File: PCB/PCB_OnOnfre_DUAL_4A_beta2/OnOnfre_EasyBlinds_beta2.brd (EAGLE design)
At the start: 44.4 x 46 mm, 27 parts, among them J3Y S8050, J7 8p, K1 OMRON-G3MB-202P-SSR2, K2 OMRON-G3MB-202P-SSR2, U2 esp12

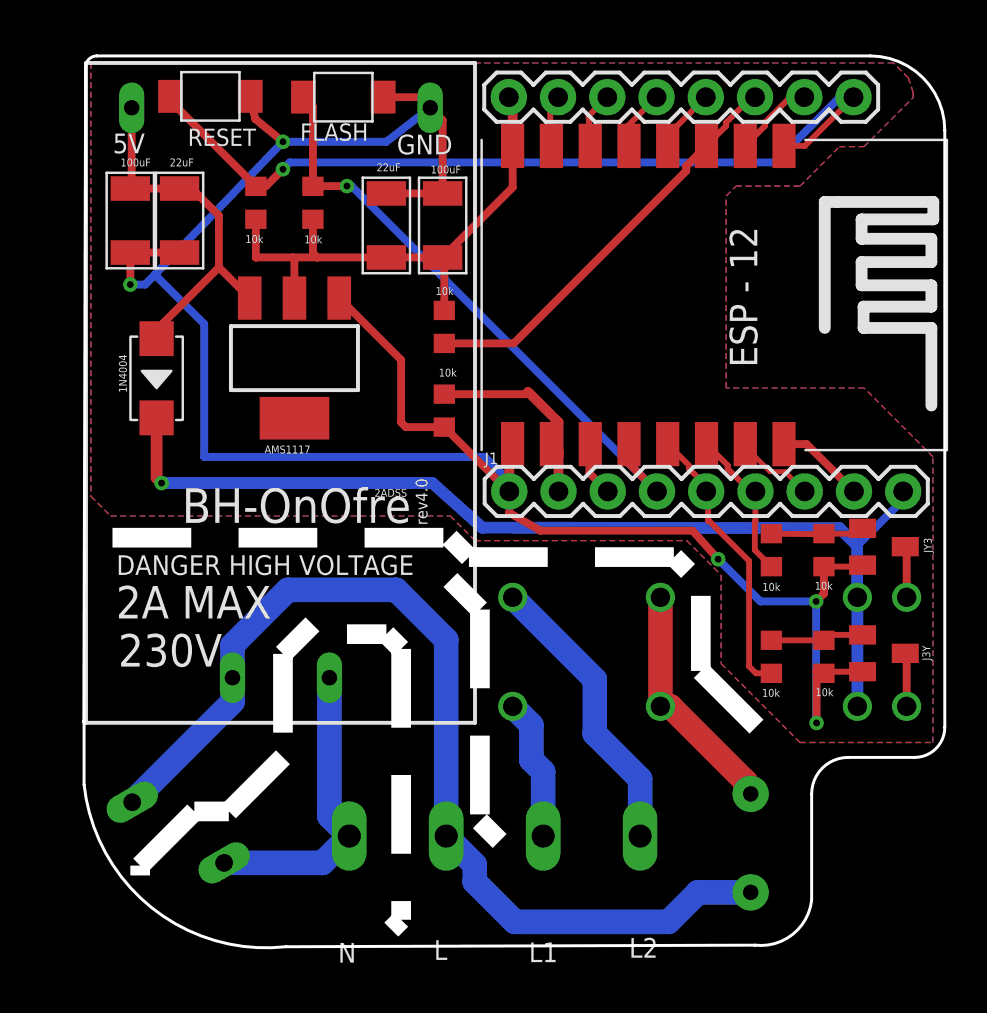
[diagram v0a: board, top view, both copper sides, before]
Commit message: beta2 board 5A
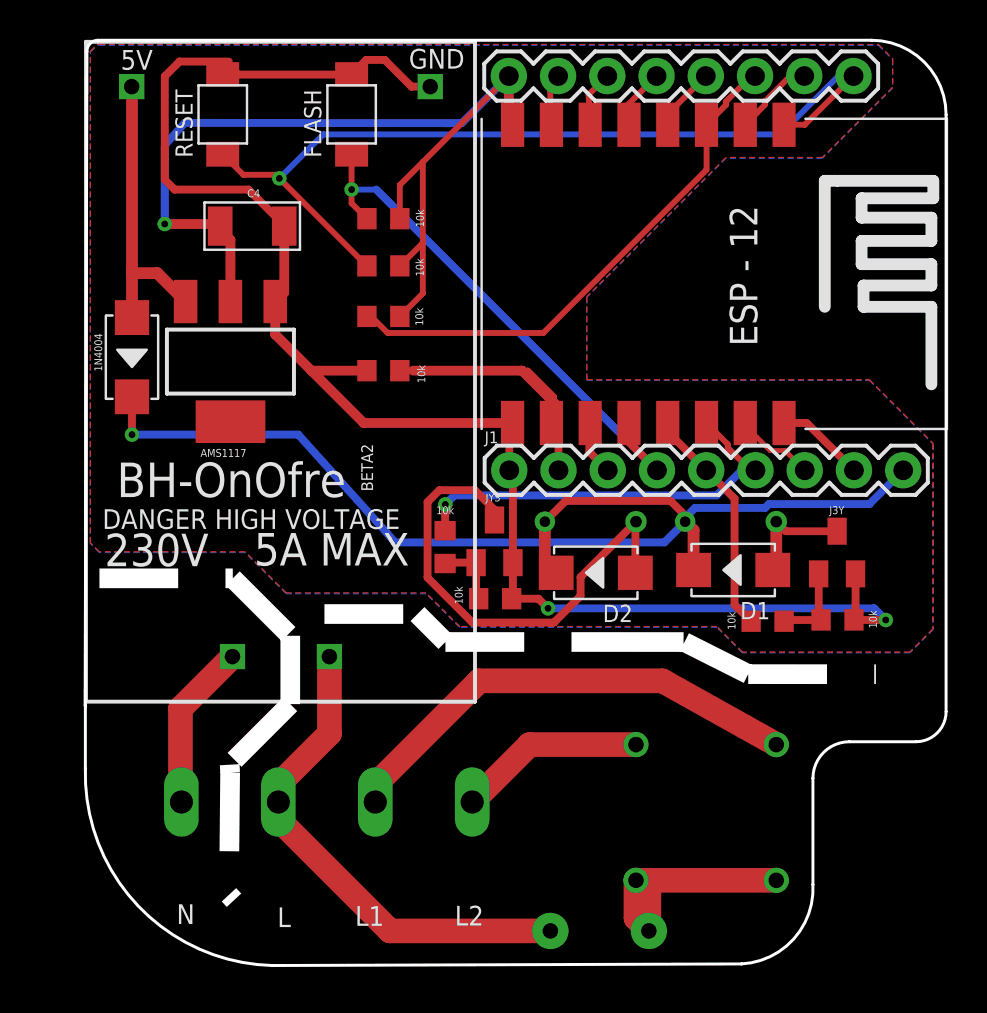
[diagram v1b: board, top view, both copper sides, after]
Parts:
- removed C1, C2: 22uF, Seeed-Capacitor:C1206
- removed C3: 100uF, Seeed-Capacitor:C1206
- removed K1, K2: OMRON-G3MB-202P-SSR2, Omron G3MB 202p SSR:OMRON-G3MB-202P-SSR
- removed R5: VARISTORS07K230, varistor:S07K230
- added D1, D2: 1N4007, Seeed-Diode:DO-214AC
- added U$1, U$3: HF46F, HF46F:HF46F
- C4: value 100uF -> 100NF
- F1: value FUSE 2A -> FUSE
- moved JY3 20.1 mm to (21.6, 21.3), turned to 0 degrees
- moved R2 17.1 mm to (21.6, 18.3), turned to 180 degrees
- moved R1 16.8 mm to (19.0, 21.0), turned to 270 degrees
- moved C4 9.82 mm to (9.08, 37.6), turned to 0 degrees
- moved F1 9.01 mm to (27.0, 1.20), turned to 180 degrees
- moved X1 8.84 mm to (12.9, 6.58)
- moved R10 7.34 mm to (15.8, 35.5), turned to 0 degrees
- moved J3Y 5.73 mm to (39.3, 20.7), turned to 0 degrees
- moved R11 3.76 mm to (15.8, 30.1), turned to 180 degrees
- moved R8 3.72 mm to (15.8, 37.9), turned to 0 degrees
- moved AMS1117 3.31 mm to (7.96, 30.6)
- moved R9 3.19 mm to (15.8, 32.9), turned to 0 degrees
- moved R3 2.02 mm to (39.3, 17.2), turned to 180 degrees
- moved R4 1.85 mm to (35.7, 17.2), turned to 0 degrees
- moved D3 1.67 mm to (2.88, 30.8)
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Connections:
- removed net FASE_IN: R5.1, U$2.P$1, X1.1
- new net LINE_IN: U$2.P$2, X1.1
- net 3V3: no longer C1.1
- net 5V: now also D1.2, D2.2, U$1.C1, U$3.C1; no longer K1.3, K2.3
- net GND: no longer C1.2, C2.2, C3.2
- net N$1: now also D1.1, U$1.C2; no longer K1.4
- net N$9: now also D2.1, U$3.C2; no longer K2.4
- net NEUTRAL_IN: now also U$2.P$1; no longer R5.2, U$2.P$2
- net NEUTRAL_IN_FUSED: now also U$1.L1, U$3.L1; no longer K1.2, K2.2
- net NEUTRAL_ONE_OUT: now also U$1.L2; no longer K1.1
- net NEUTRAL_TWO_OUT: now also U$3.L2; no longer K2.1
- net VCC: no longer C2.1, C3.1
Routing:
- net GND: track 115.9 -> 84.6 mm, vias 5 -> 2
- net NEUTRAL_IN: track 52.3 -> 25.9 mm
- net N$9: track 2.64 -> 25.6 mm
- net 3V3: track 30.7 -> 52.8 mm, vias 0 -> 1
- net NEUTRAL_ONE_OUT: track 7.34 -> 24.7 mm
- net FASE_IN: track 15.6 -> 0.00 mm
- net GPIO05: track 7.89 -> 21.7 mm, vias 0 -> 1
- net LINE_IN: track 0.00 -> 9.37 mm
- net 5V: track 52.7 -> 59.7 mm
- net GPIO0: track 34.6 -> 28.7 mm
- net CH_PD: track 21.5 -> 27.3 mm
- net NEUTRAL_TWO_OUT: track 15.0 -> 9.67 mm
- net VCC: track 19.3 -> 15.3 mm
- net N$1: track 2.76 -> 5.91 mm
- net GPIO04: track 14.7 -> 12.0 mm
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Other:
- board size 44.4 x 46 mm -> 44.4 x 47.7 mm
- board text added: "5A MAX"
- board text added: "BETA2"
- board text removed: "2A MAX"
- board text removed: "2ADSS"
- board text removed: "rev4.0"
